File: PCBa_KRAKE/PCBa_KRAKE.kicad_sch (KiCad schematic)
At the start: 94 parts, among them J101 Barrel_Jack_Switch_SMT, J102 0.100_2Pin, J103 0.100_2Pin, J105 S04B-XASK-1(LF)(SN)Rev2, U1 AMS1117-3.3, U101 LM7805_TO220, U102 PI_ATMEGA328P-AU-InOrder, U999 ESP32-WROOM-32D

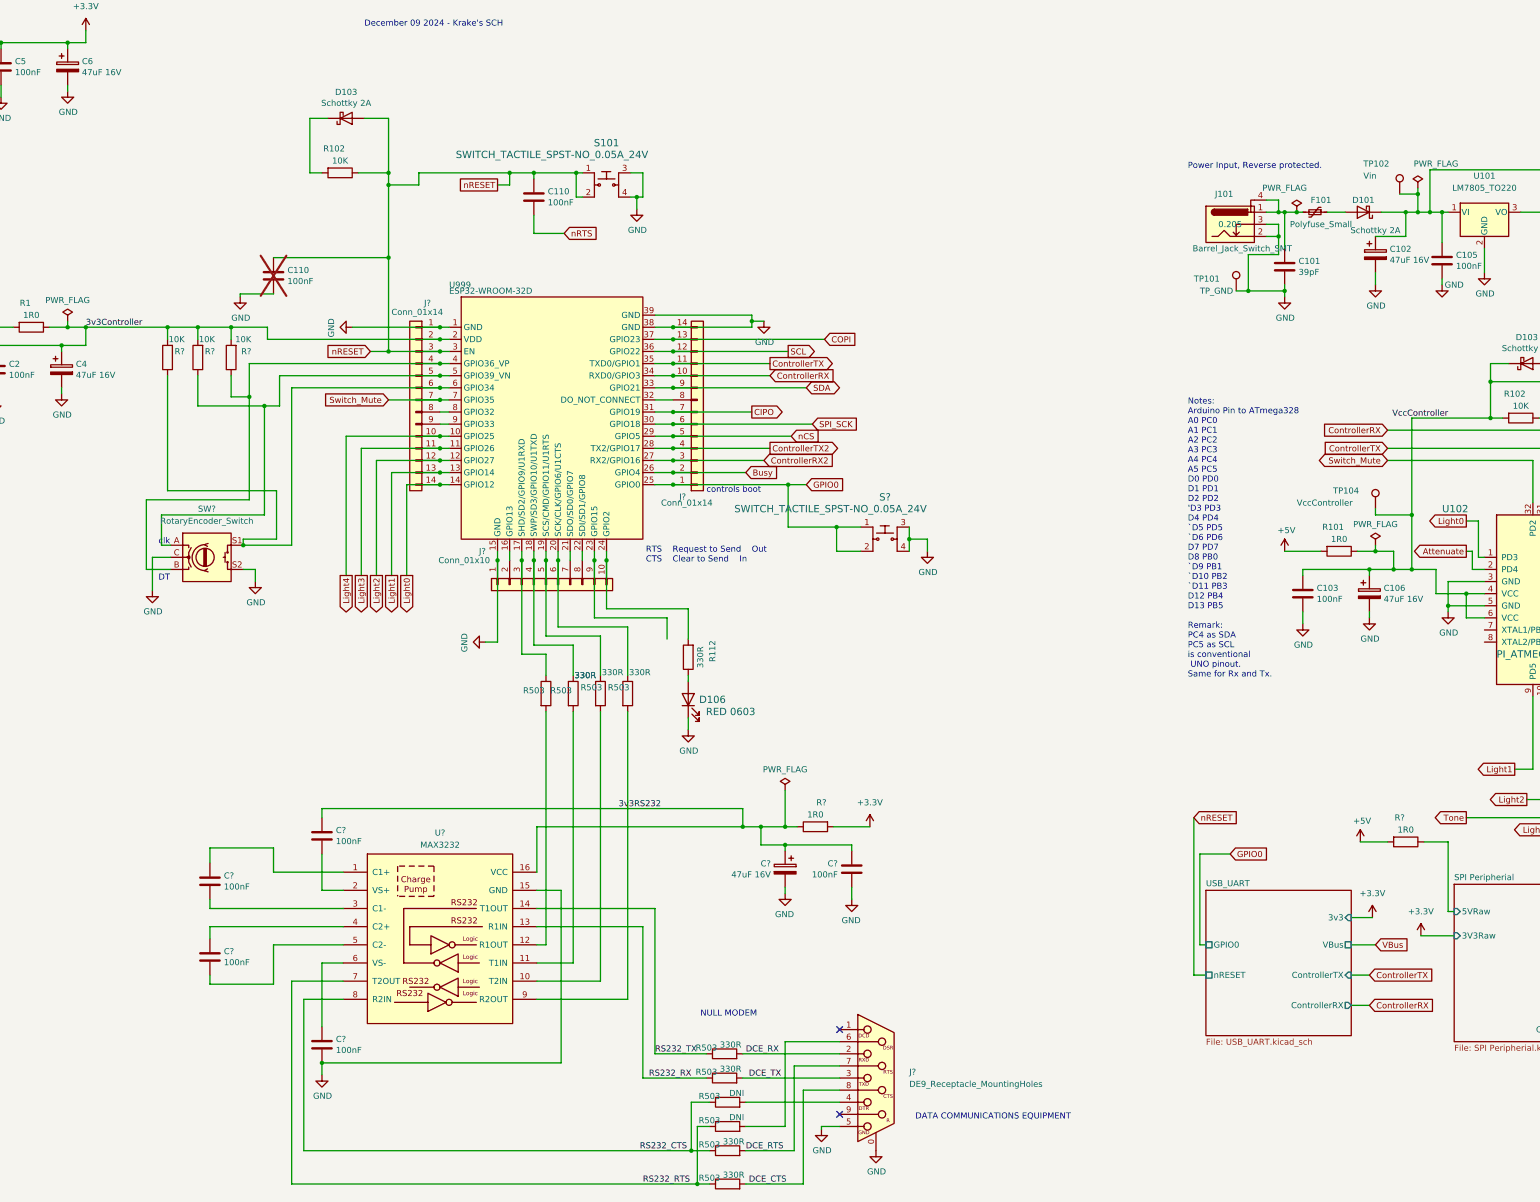
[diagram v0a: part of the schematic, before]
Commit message: Replaced USB B with USB C connector.
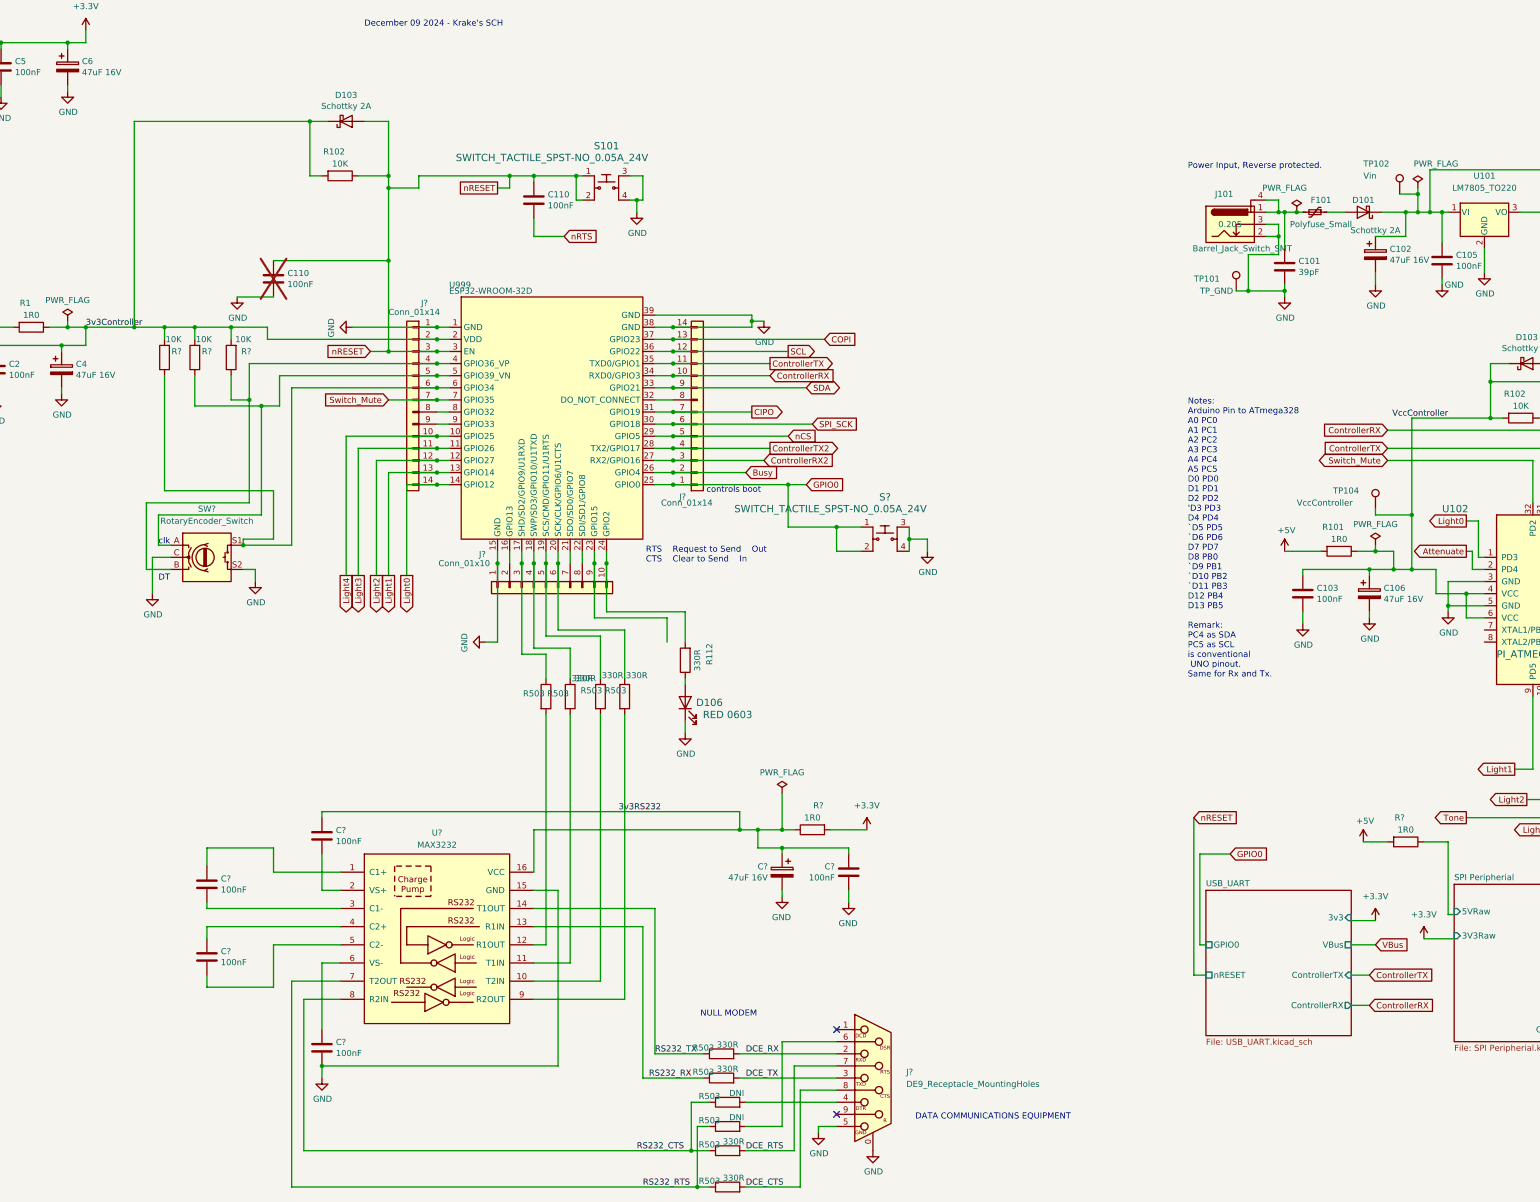
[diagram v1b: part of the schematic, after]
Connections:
- net 3v3Controller: now also D103.1 (K), R102.2
- net SPI Peripherial/5VRaw: no longer R?.1
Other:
- moved on the sheet: C110, C?, D103, D106, J?, R102, R112, R503, R?, S101, U?

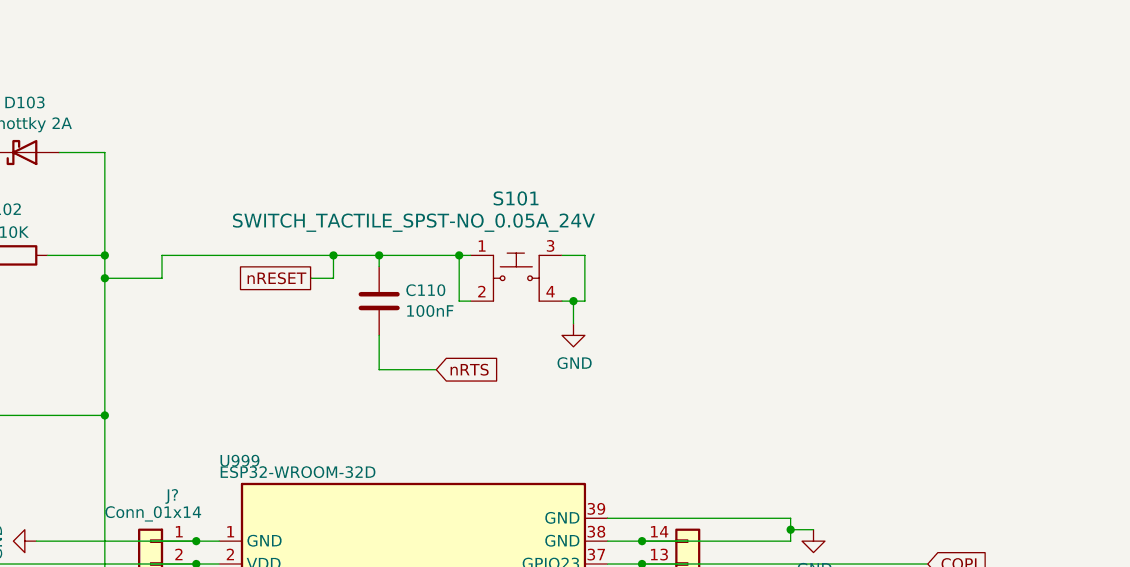
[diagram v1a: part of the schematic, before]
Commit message: Finalized the nRESET circuit.
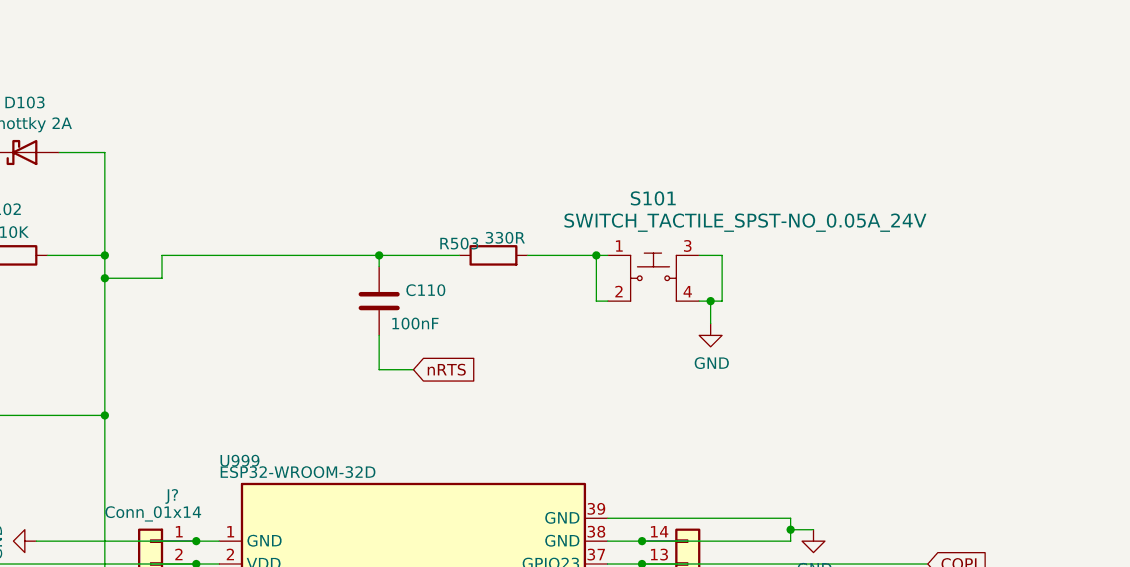
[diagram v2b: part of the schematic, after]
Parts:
- added R503: 330R, Resistor_SMD:R_0603_1608Metric_Pad0.98x0.95mm_HandSolder, symbol Device:R
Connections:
- net nRESET: now also R503.1; no longer S101.1, S101.2
- new net: R503.2, S101.1, S101.2
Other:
- moved on the sheet: S101

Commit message: Deleting the I2C ciruit.
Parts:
- removed C113, C114: 39pF, Capacitor_SMD:C_0603_1608Metric_Pad1.08x0.95mm_HandSolder, symbol Device:C
- removed J105: S04B-XASK-1(LF)(SN)Rev2, GeneralPurposeAlarmDevicePCB:S04B-XASK-1(LF)(SN)Rev2, symbol GPAD_SCH_LIB:S04B-XASK-1(LF)(SN)Rev2
- removed R104, R105: 39R, Resistor_SMD:R_0603_1608Metric_Pad0.98x0.95mm_HandSolder, symbol Device:R
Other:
- note removed: "December 09 2024 - Krake's SCH"

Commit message: removed ATMEGA328P and replaced it with ESP32. Added a hierarchial sheet for the RS232.
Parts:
- removed C103, C110, C111, C? (x5): 100nF, Capacitor_SMD:C_0603_1608Metric_Pad1.08x0.95mm_HandSolder, symbol Device:C
- removed C106, C112, C?: 47uF 16V, Capacitor_SMD:CP_Elec_5x5.4, symbol Device:C_Polarized
- removed D102, D106: RED 0603, LED_SMD:LED_0603_1608Metric_Pad1.05x0.95mm_HandSolder, symbol Device:LED
- removed D103: Schottky 2A, Diode_SMD:D_SMB, symbol Device:D_Schottky
- removed J?: DE9_Receptacle_MountingHoles, Connector_Dsub:DSUB-9_Female_Horizontal_P2.77x2.84mm_EdgePinOffset9.90mm_Housed_MountingHolesOffset11.32mm, symbol GPAD_SCH_LIB:DE9_Receptacle_MountingHoles_wSIGNALnames
- removed R101, R?: 1R0, Resistor_SMD:R_0603_1608Metric_Pad0.98x0.95mm_HandSolder, symbol Device:R
- removed R102: 10K, Resistor_SMD:R_0603_1608Metric_Pad0.98x0.95mm_HandSolder, symbol Device:R
- removed R103, R503 (x2): DNI, Resistor_SMD:R_0603_1608Metric_Pad0.98x0.95mm_HandSolder, symbol Device:R
- removed R108, R109: 1K, Resistor_SMD:R_0603_1608Metric_Pad0.98x0.95mm_HandSolder, symbol Device:R
- removed R112, R503 (x8): 330R, Resistor_SMD:R_0603_1608Metric_Pad0.98x0.95mm_HandSolder, symbol Device:R
- removed S101: SWITCH_TACTILE_SPST-NO_0.05A_24V, GeneralPurposeAlarmDevicePCB:Switch_Tactile_THT_6x6mm, symbol GPAD_SCH_LIB:SWITCH_TACTILE_SPST-NO_0.05A_24V
- removed TP104: VccController, TestPoint:TestPoint_Loop_D2.54mm_Drill1.5mm_Beaded, symbol Connector:TestPoint
- removed TP105: 3.3V, TestPoint:TestPoint_Loop_D2.54mm_Drill1.5mm_Beaded, symbol Connector:TestPoint
- removed U102: PI_ATMEGA328P-AU-InOrder, Package_QFP:TQFP-32_7x7mm_P0.8mm, symbol GPAD_SCH_LIB:PI_ATMEGA328P-AU-InOrder
- removed U?: MAX3232, Package_SO:SOIC-16_4.55x10.3mm_P1.27mm, symbol GPAD_SCH_LIB:MAX3232_InOrder
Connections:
- net RX0: now reaches J?.3 (Pin_3), U999.17 (SHD/SD2/GPIO9/U1RXD)
- net TX0: now reaches J?.4 (Pin_4), U999.18 (SWP/SD3/GPIO10/U1TXD)
- net RTS: now reaches J?.5 (Pin_5), U999.19 (SCS/CMD/GPIO11/U1RTS)
- net CTS: now reaches J?.6 (Pin_6), U999.20 (SCK/CLK/GPIO6/U1CTS)
- no-connect marks 4 -> 0
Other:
- added sheet RS232 (RS232.kicad_sch)
- note removed: "DATA COMMUNICATIONS EQUIPMENT"
- note removed: "NULL MODEM"
- note removed: "Note: Using 0603HandSolder for Rs and Cs."
- note removed: "Notes: Arduino Pin to ATmega328 A0 PC0 A1 PC1 A2 PC2 A3 PC3 A4 PC4 A5 PC5 D0 PD0 D1 PD1 D2 PD2 'D3 PD3 D4 PD4 `D5 PD5 `D6 PD6 D7 PD7 D8 PB0 `D9 PB1 `D10 PB2 `D11 PB3 D12 PB4 D13 PB5 Remark: PC4 as SDA PC5 as SCL is conventional UNO pinout. Same for Rx and Tx."
- note removed: "UNO Headers"
- note removed: "Wink LED"
- moved on the sheet: C1, C110, C2, C3, C4, C5, C6, D103, D106, H101, H102, H103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

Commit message: Adding global labels RS232. Adding Enclosure hierarchial page.
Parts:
- removed MF101: PCB_GPAD_VER2, NA, symbol GPAD_SCH_LIB:PCB_GPAD_VER1
- removed MF102: ENCLOSURE_GPAD_VER1, symbol GPAD_SCH_LIB:ENCLOSURE_GPAD_VER1
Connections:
- net SPI Peripherial/5VRaw: now also R?.1
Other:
- added sheet Enclosure Sheet (Enclosure.kicad_sch)
- sheet RS232 ports: added CTS, RTS, RX0, TX0; removed none
- moved on the sheet: D106, R112

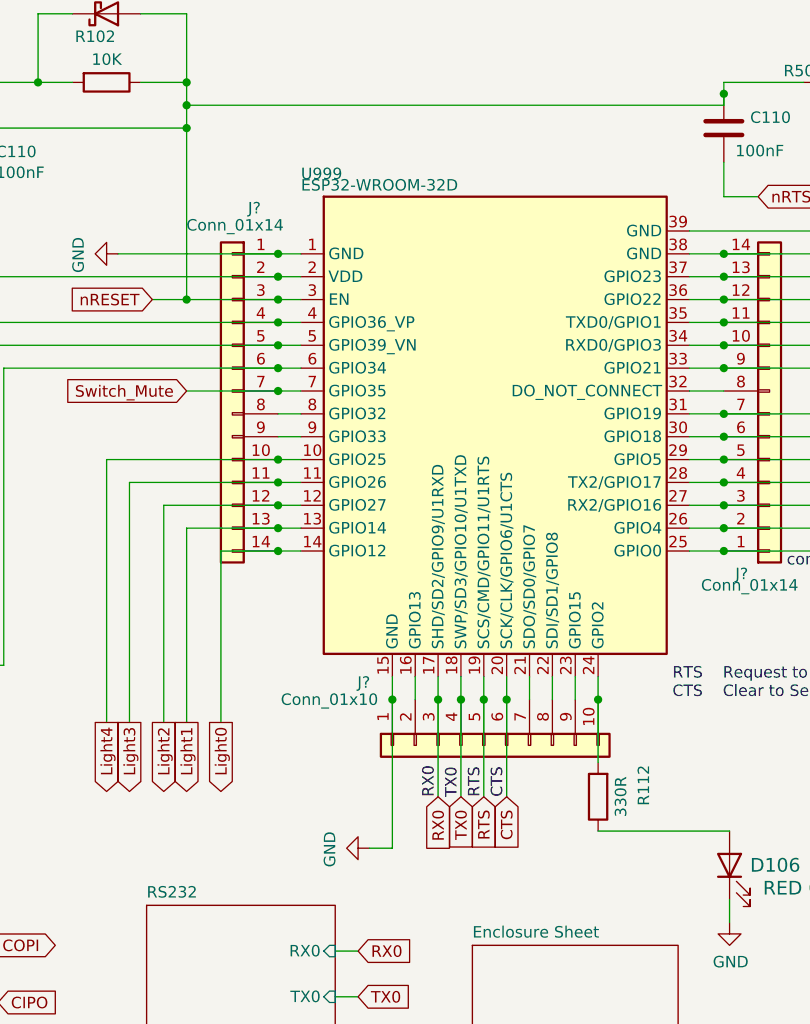
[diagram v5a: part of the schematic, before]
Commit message: Corrected UART1 labels. Renamed Esp32 as U102.
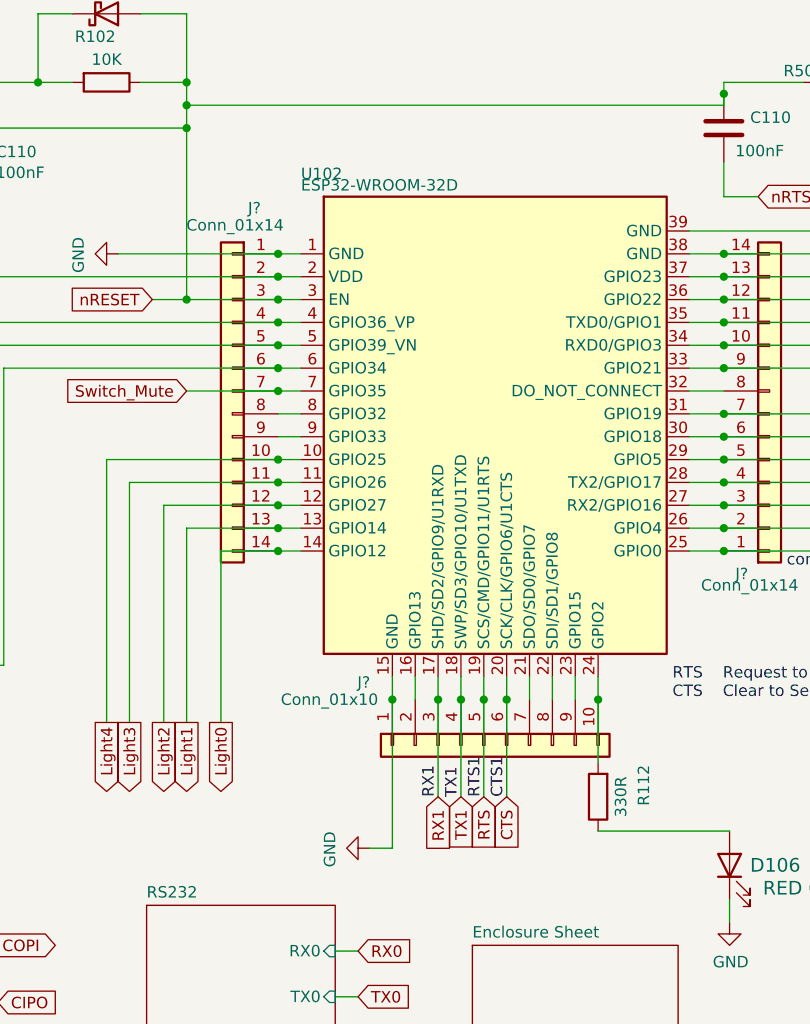
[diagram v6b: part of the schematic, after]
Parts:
- renumbered U999 to U102
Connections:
- net RX0: no longer J?.3 (Pin_3), U102.17 (SHD/SD2/GPIO9/U1RXD)
- net TX0: no longer J?.4 (Pin_4), U102.18 (SWP/SD3/GPIO10/U1TXD)
- new net RX1: J?.3 (Pin_3), U102.17 (SHD/SD2/GPIO9/U1RXD)
- new net TX1: J?.4 (Pin_4), U102.18 (SWP/SD3/GPIO10/U1TXD)
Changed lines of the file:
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@@
     (effects (font (size 1.27 1.27)) (justify left bottom))
   )
-  (label "CTS" (at 149.225 151.13 90) (fields_autoplaced)
+  (label "CTS1" (at 149.225 151.13 90) (fields_autoplaced)
     (effects (font (size 1.27 1.27)) (justify left bottom))
   )
-  (label "TX0" (at 144.145 151.13 90) (fields_autoplaced)
+  (label "TX1" (at 144.145 151.13 90) (fields_autoplaced)
     (effects (font (size 1.27 1.27)) (justify left bottom))
   )
@@
     (effects (font (size 1.27 1.27)) (justify left bottom))
   )
-  (label "RTS" (at 146.685 151.13 90) (fields_autoplaced)
+  (label "RTS1" (at 146.685 151.13 90) (fields_autoplaced)
     (effects (font (size 1.27 1.27)) (justify left bottom))
   )
-  (label "RX0" (at 141.605 151.13 90) (fields_autoplaced)
+  (label "RX1" (at 141.605 151.13 90) (fields_autoplaced)
     (effects (font (size 1.27 1.27)) (justify left bottom))
   )
@@
     )
   )
-  (global_label "TX0" (shape input) (at 144.145 151.13 270) (fields_autoplaced)
+  (global_label "TX1" (shape input) (at 144.145 151.13 270) (fields_autoplaced)
     (effects (font (size 1.27 1.27)) (justify right))
     (property "Intersheetrefs" "${INTERSHEET_REFS}" (at 144.145 156.7682 90)
@@
     )
   )
-  (global_label "RX0" (shape input) (at 141.605 151.13 270) (fields_autoplaced)
+  (global_label "RX1" (shape input) (at 141.605 151.13 270) (fields_autoplaced)
     (effects (font (size 1.27 1.27)) (justify right))
     (property "Intersheetrefs" "${INTERSHEET_REFS}" (at 141.605 157.0706 90)
@@
   (symbol (lib_id "GPAD_SCH_LIB:ESP32-WROOM-32D-PINORDER") (at 147.955 111.125 0) (unit 1)
     (in_bom yes) (on_board yes) (dnp no)
-    (property "Reference" "U999" (at 126.365 81.915 0)
+    (property "Reference" "U102" (at 126.365 81.915 0)
       (effects (font (size 1.27 1.27)) (justify left))
     )
@@
       (project "PCBa_KRAKE"
         (path "/412a327d-1ee3-473e-bc00-1545004b7edf"
-          (reference "U999") (unit 1)
-        )
-      )
+          (reference "U102") (unit 1)
+        )
+      )
